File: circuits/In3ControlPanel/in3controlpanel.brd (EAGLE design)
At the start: 47.5 x 42 mm, 27 parts, among them IC1 ATMEGA48/88/168-AU, SW1 EC12E_SW

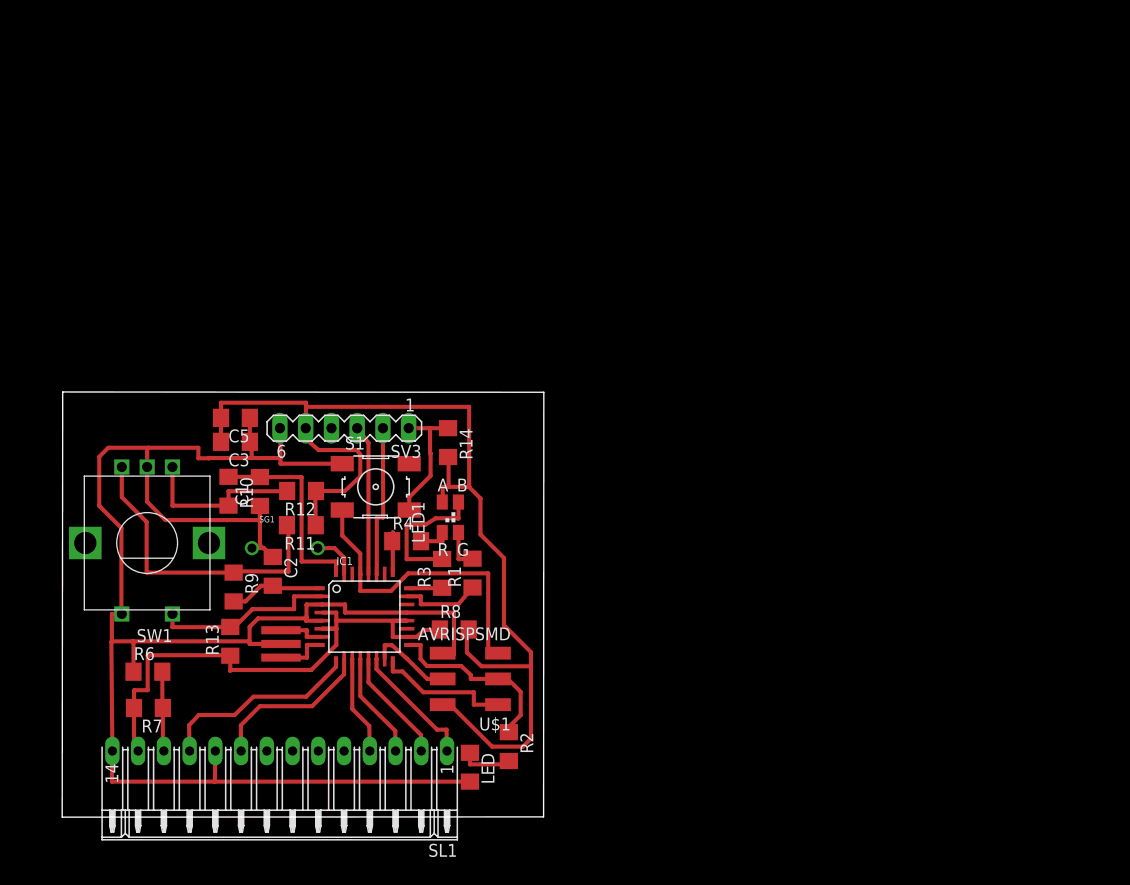
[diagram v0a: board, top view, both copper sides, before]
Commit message: Electronics v2
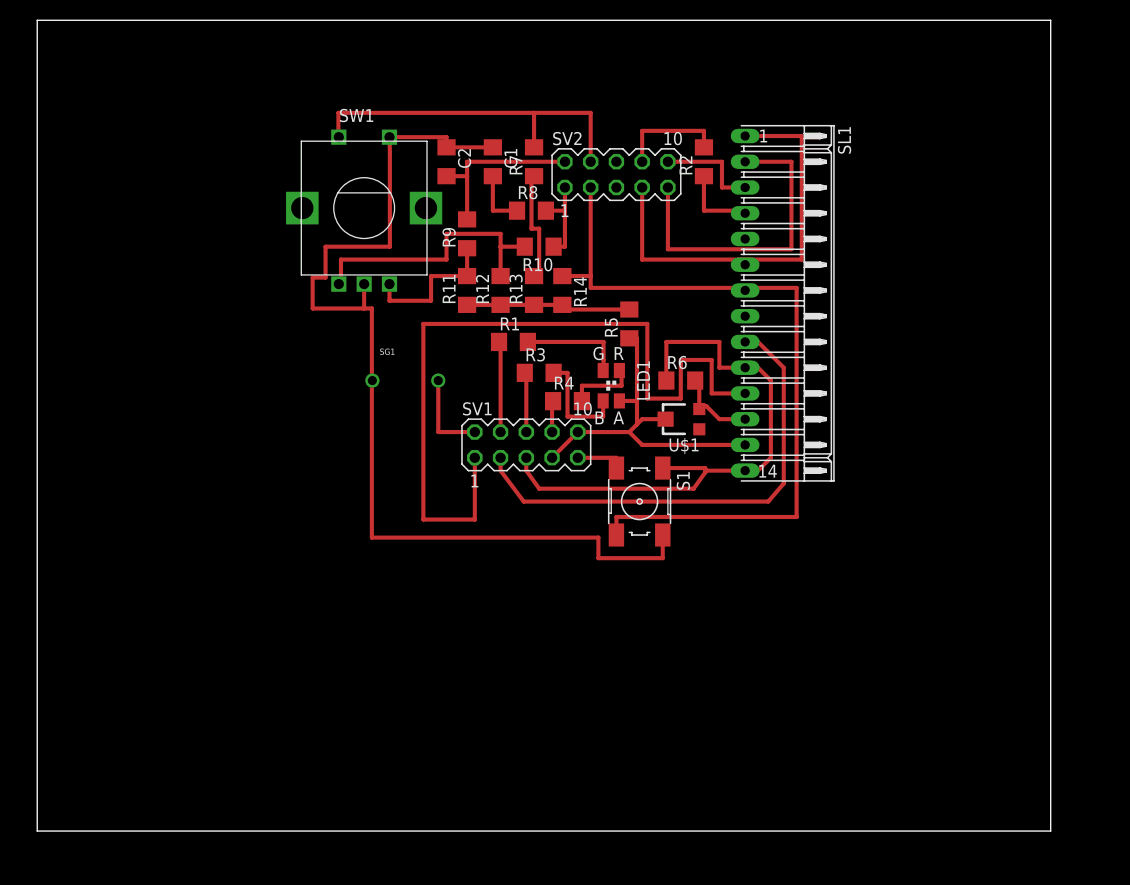
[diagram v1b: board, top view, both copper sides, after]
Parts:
- removed C3: .1uf, ng:1206
- removed C5: 10uf, ng:1206
- removed IC1: ATMEGA48/88/168-AU, atmega8:TQFP32-08
- removed LED: (no value), ng:1206
- removed SV3: (no value), con-lstb:MA06-1
- removed U$2: RESONATOREFOB, fab:EFOBM
- added R5: 0, ng:1206
- added SV1, SV2: (no value), con-lstb:MA05-2
- C1, C2: value (none) -> 0.01uf
- R2: value 499 -> 0
- R7: value 1k -> 0
- U$1: value AVRISPSMD -> (none); device 01_FAB_Hello:2X03SMD -> 01_adafruit:TC33X
- moved R7 66.0 mm to (49.0, 66.0), turned to 90 degrees
- moved SL1 63.7 mm to (69.8, 52.1), turned to 270 degrees
- moved R2 60.8 mm to (65.8, 66.0), turned to 90 degrees
- moved R6 59.9 mm to (63.5, 44.5)
- moved R13 45.8 mm to (49.0, 53.3)
- moved C2 43.9 mm to (40.4, 66.0)
- moved R8 42.0 mm to (48.8, 61.2)
- moved R9 41.8 mm to (42.4, 58.9), turned to 90 degrees
- moved C1 39.8 mm to (45.0, 66.0), turned to 270 degrees
- moved SW1 39.4 mm to (32.3, 61.5), turned to 0 degrees
- moved R10 39.0 mm to (49.5, 57.7), turned to 180 degrees
- moved U$1 32.9 mm to (63.5, 40.6), turned to 90 degrees
- moved R11 28.4 mm to (42.4, 53.3), turned to 90 degrees
- moved R12 27.9 mm to (45.7, 53.3), turned to 90 degrees
- moved S1 26.1 mm to (59.4, 32.5), turned to 270 degrees
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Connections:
- removed net 12V: SV3.4
- removed net ADC6: IC1.19
- removed net MISO: IC1.16, U$1.1
- removed net MOSI: IC1.15, U$1.4
- removed net N$1: IC1.8, U$2.1
- removed net N$23: LED.1, R2.2
- removed net N$9: IC1.7, U$2.3
- removed net PB0: IC1.12, SL1.3
- removed net PB1: IC1.13, SL1.2
- removed net PB2: IC1.14, SL1.1
- removed net PC0: IC1.23, R1.1
- removed net PC1: IC1.24, R3.1
- removed net PC2: IC1.25, R4.1
- removed net PD0: IC1.30
- removed net PD1: IC1.31, SG1.+
- removed net PD5: IC1.9, SL1.11
- removed net PD6: IC1.10, SL1.9
- removed net PD7: IC1.11, SL1.4
- removed net SCL: IC1.28, SV3.3
- removed net SDA: IC1.27, SV3.2
- removed net SWBUTTON: IC1.2, R13.2, SW1.D
- new net $1: SV2.5
- new net $2: SV2.6
- new net BTN: R13.2, R7.1, R7.2, SV2.4, SW1.D
- new net BUZZ: SG1.+, SV1.2
- new net LCD4: R2.1, R2.2, SL1.4, SV2.8
- new net LCD5: SL1.3, SV2.10
- new net LCD6: SL1.2, SV2.9
- new net LCD7: SL1.1, SV2.7
- new net LCDE: SL1.9, SV1.3
- new net LCDRS: SL1.11, SV1.1
- new net RGBB: R3.1, SV1.6
- new net RGBG: R1.1, SV1.4
- net 5V: now also R5.1, R5.2, SV1.10, SV1.7; no longer C3.2, C5.2, IC1.18, IC1.20, IC1.4, IC1.6, R7.2, R8.1, R8.2, SV3.5
- net GND: now also S1.2, SV1.5; no longer C3.1, C5.1, IC1.21, IC1.3, IC1.5, LED.2, SV3.6, U$1.6, U$2.2
- net INT0: now also R8.1, R8.2, SV2.1; no longer IC1.32
- net INT1: now also SV2.2; no longer IC1.1
- net N$6: now also U$1.3; no longer R7.1
- net RST: now also SV1.9, SV2.3; no longer IC1.29, SV3.1, U$1.5
- net SCK: now also R4.1, SV1.8; no longer IC1.17, R2.1, U$1.3
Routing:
- net 5V: track 166.4 -> 52.2 mm
- net LCDRS: track 0.00 -> 76.7 mm
- net BTN: track 0.00 -> 47.9 mm
- net LCDE: track 0.00 -> 47.8 mm
- net LCD7: track 0.00 -> 40.6 mm
- net RST: track 43.9 -> 80.0 mm
- net LCD6: track 0.00 -> 31.5 mm
- net GND: track 182.7 -> 157.0 mm
- net PD5: track 20.0 -> 0.00 mm
- net LCD4: track 0.00 -> 18.5 mm
- net SWBUTTON: track 18.1 -> 0.00 mm
- net PD6: track 16.3 -> 0.00 mm
- net N$5: track 30.5 -> 14.5 mm
- net SCK: track 18.4 -> 3.15 mm
- net SDA: track 15.1 -> 0.00 mm
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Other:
- board size 47.5 x 42 mm -> 100 x 80 mm

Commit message: New Electronics
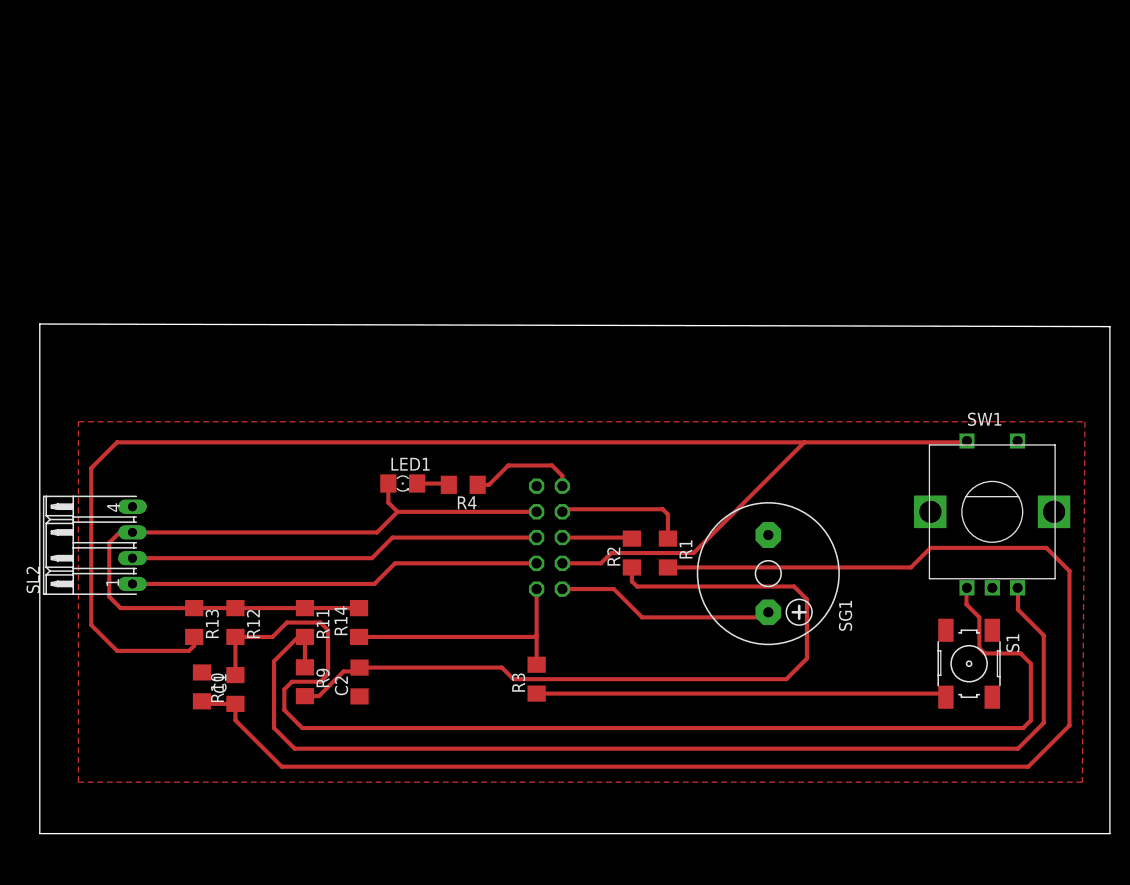
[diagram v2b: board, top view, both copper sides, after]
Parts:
- removed R5, R7, R8: 0, ng:1206
- removed R6: 10k, ng:1206
- removed SL1: (no value), con-amp-quick:14PA
- removed SV1: (no value), con-lstb:MA05-2
- removed U$1: (no value), 01_adafruit:TC33X
- added SL2: (no value), con-amp-quick:04PA
- LED1: device 01_fab:P-LCC-4-3 -> eagle-ltspice:LED_1206
- R1: value 1k -> 0R
- R3: value 470 -> 0
- SG1: value BUZZERNS -> F/CM12P; device 01_SparkFun:BUZZER-12MM-NS -> buzzer:F/CM12P
- moved SW1 68.8 mm to (94.2, 31.5)
- moved C1 59.2 mm to (16.3, 14.2)
- moved R10 53.0 mm to (19.6, 14.0), turned to 90 degrees
- moved C2 52.0 mm to (31.8, 14.7), turned to 90 degrees
- moved R9 47.0 mm to (26.4, 14.7), turned to 270 degrees
- moved R13 46.9 mm to (15.5, 20.6), turned to 270 degrees
- moved R12 41.9 mm to (19.6, 20.6), turned to 270 degrees
- moved SG1 40.6 mm to (72.1, 25.4), turned to 270 degrees
- moved R2 39.3 mm to (58.7, 27.4)
- moved R14 38.4 mm to (31.8, 20.6), turned to 90 degrees
- moved R11 36.5 mm to (26.4, 20.6), turned to 270 degrees
- moved SV2 36.4 mm to (50.5, 29.0), flipped to the bottom, turned to 90 degrees
- moved S1 36.2 mm to (91.9, 16.5)
- moved R3 30.2 mm to (49.3, 15.0), turned to 90 degrees
- moved R1 25.8 mm to (62.2, 27.4), turned to 270 degrees
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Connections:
- removed net $1: SV2.5
- removed net $2: SV2.6
- removed net LCD4: R2.1, R2.2, SL1.4, SV2.8
- removed net LCD5: SL1.3, SV2.10
- removed net LCD6: SL1.2, SV2.9
- removed net LCD7: SL1.1, SV2.7
- removed net LCDE: SL1.9, SV1.3
- removed net LCDRS: SL1.11, SV1.1
- removed net N$2: LED1.G, R1.2
- removed net N$3: LED1.B, R3.2
- removed net N$4: LED1.R, R4.2
- removed net N$6: R6.2, SL1.12, U$1.3
- removed net RGBB: R3.1, SV1.6
- removed net RGBG: R1.1, SV1.4
- removed net SCK: R4.1, SV1.8
- new net LED: R4.1, SV2.10
- new net N$1: LED1.C, R4.2
- new net SCL: SL2.1, SV2.3
- new net SDA: SL2.2, SV2.5
- net 5V: now also SL2.3, SV2.7; no longer R5.1, R5.2, SL1.13, SV1.10, SV1.7, U$1.2
- net BTN: no longer R7.1, R7.2
- net BUZZ: now also SV2.2; no longer SV1.2
- net GND: now also SL2.4, SV2.9; no longer R6.1, SL1.10, SL1.14, SV1.5
- net INT0: now also R1.1, R1.2, SV2.8; no longer R8.1, R8.2, SV2.1
- net INT1: now also R2.1, R2.2, SV2.6; no longer SV2.2
- net RST: now also R3.1, R3.2, SV2.1; no longer SV1.9, SV2.3
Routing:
- net GND: track 157.0 -> 0.00 mm
- net INT0: track 14.6 -> 161.7 mm
- net BTN: track 47.9 -> 144.1 mm
- net N$5: track 14.5 -> 105.9 mm
- net N$8: track 27.5 -> 117.6 mm
- net LCDRS: track 76.7 -> 0.00 mm
- net INT1: track 17.4 -> 84.1 mm
- net LCDE: track 47.8 -> 0.00 mm
- net SDA: track 0.00 -> 40.7 mm
- net SCL: track 0.00 -> 40.7 mm
- net LCD7: track 40.6 -> 0.00 mm
- net LCD6: track 31.5 -> 0.00 mm
- net 5V: track 52.2 -> 77.0 mm
- net LCD4: track 18.5 -> 0.00 mm
- net RST: track 80.0 -> 66.4 mm
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- added copper zone on layer 1, net GND
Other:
- board size 100 x 80 mm -> 105.6 x 50.3 mm
